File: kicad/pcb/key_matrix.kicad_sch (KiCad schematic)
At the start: 38 parts, among them SW1 EC_SW, SW10 EC_SW, SW11 EC_SW, SW12 EC_SW, SW13 EC_SW, SW14 EC_SW, SW15 EC_SW, SW2 EC_SW, SW3 EC_SW, SW35 SW_Push, SW36 Rotary_Encoder_Switch, SW4 EC_SW, SW5 EC_SW, SW6 EC_SW, SW7 EC_SW, SW8 EC_SW, SW9 EC_SW

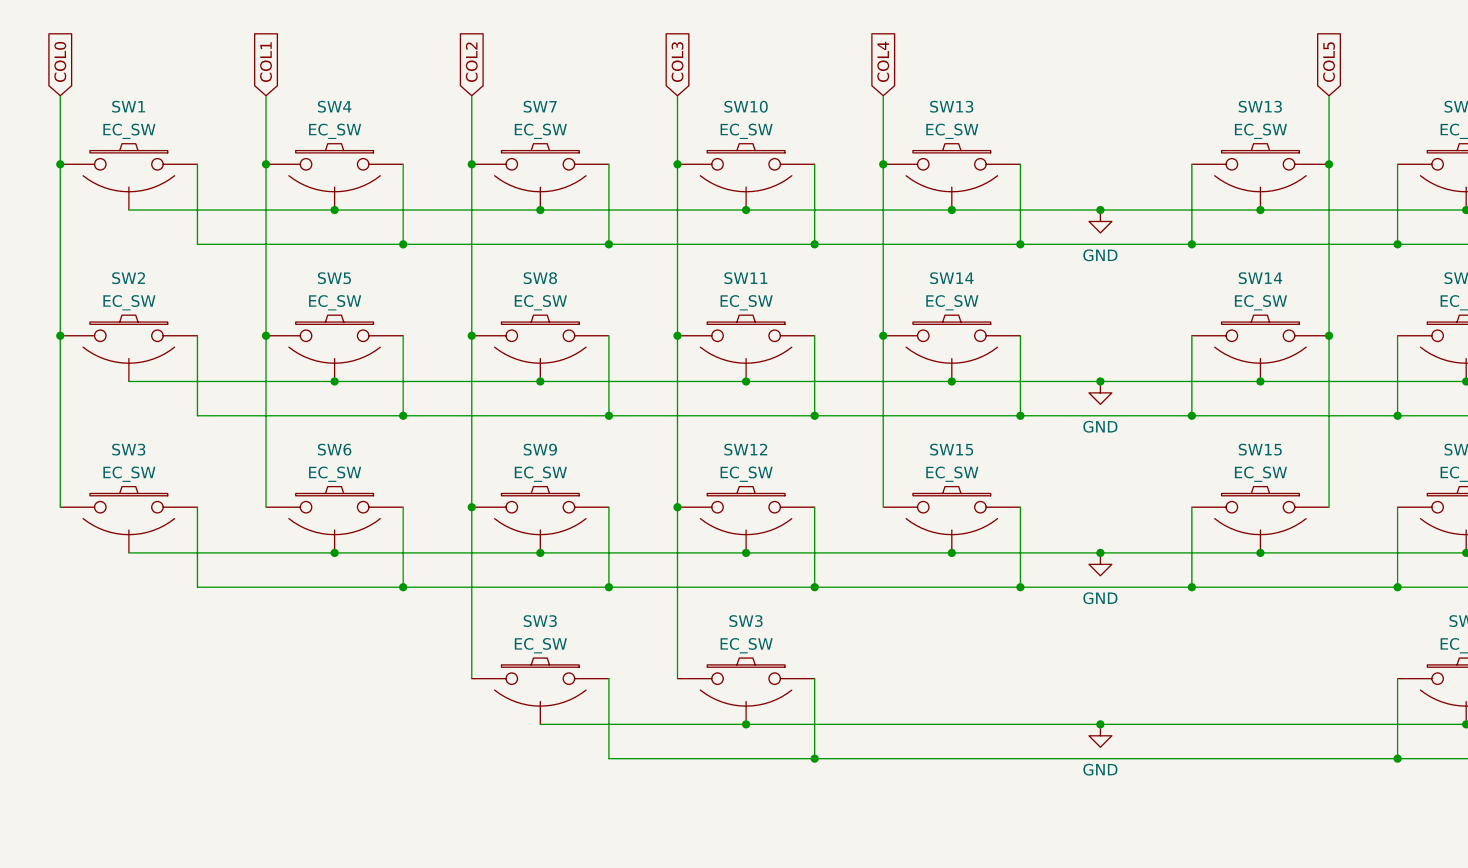
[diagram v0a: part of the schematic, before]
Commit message: rerouted pcb
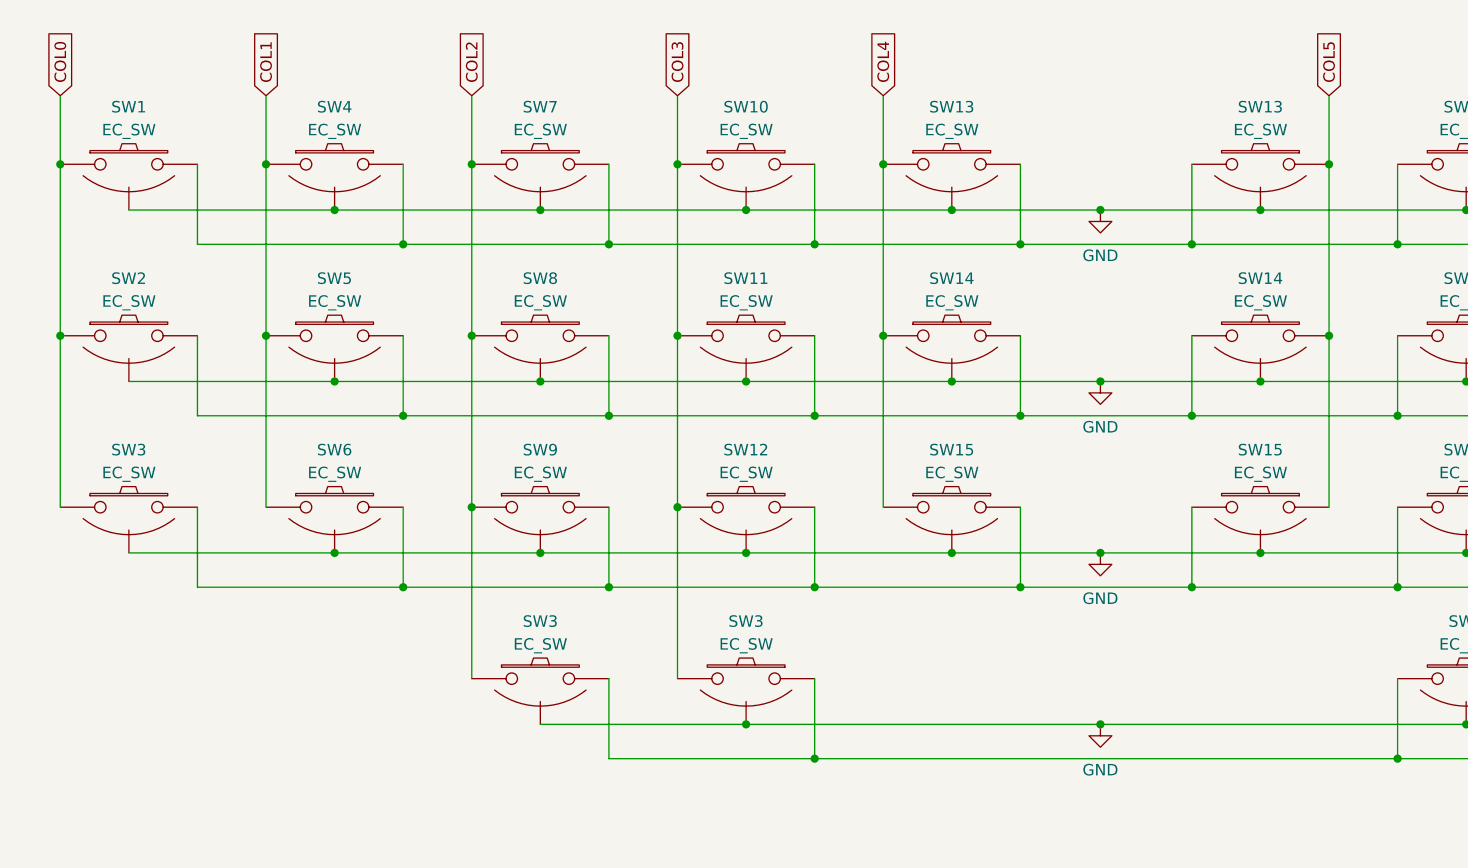
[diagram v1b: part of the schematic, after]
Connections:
- net COL0: now also SW1.1, SW2.1, SW3.1; no longer SW1.2, SW2.2, SW3.2
- net COL1: now also SW4.1, SW5.1, SW6.1; no longer SW4.2, SW5.2, SW6.2
- net COL2: now also SW3.1, SW7.1, SW8.1, SW9.1; no longer SW3.2, SW7.2, SW8.2, SW9.2
- net COL3: now also SW10.1, SW11.1, SW12.1; no longer SW10.2, SW11.2, SW12.2
- net COL4: now also SW13.1, SW14.1, SW15.1; no longer SW13.2, SW14.2, SW15.2
- net COL5: now also SW14.2; no longer SW14.1
- net ROW0: now also SW1.2, SW10.2, SW13.2, SW4.2, SW7.2; no longer SW1.1, SW10.1, SW13.1, SW4.1, SW7.1
- net ROW1: now also SW11.2, SW14.1, SW14.2, SW2.2, SW5.2, SW8.2; no longer SW11.1, SW14.1, SW14.2, SW2.1, SW5.1, SW8.1
- net ROW2: now also SW12.2, SW15.2, SW3.2, SW6.2, SW9.2; no longer SW12.1, SW15.1, SW3.1, SW6.1, SW9.1
- net ROW3: now also SW3.2; no longer SW3.1
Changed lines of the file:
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@@
     )
   )
-  (symbol (lib_id "cipulot_parts:EC_SW") (at 133.985 39.37 0) (mirror y) (unit 1)
+  (symbol (lib_id "cipulot_parts:EC_SW") (at 133.985 39.37 0) (unit 1)
     (in_bom no) (on_board yes) (dnp no)
     (property "Reference" "SW13" (at 133.985 33.02 0)
@@
     )
   )
-  (symbol (lib_id "cipulot_parts:EC_SW") (at 133.985 58.42 0) (mirror y) (unit 1)
+  (symbol (lib_id "cipulot_parts:EC_SW") (at 133.985 58.42 0) (unit 1)
     (in_bom no) (on_board yes) (dnp no)
     (property "Reference" "SW14" (at 133.985 52.07 0)
@@
     )
   )
-  (symbol (lib_id "cipulot_parts:EC_SW") (at 65.405 58.42 0) (mirror y) (unit 1)
+  (symbol (lib_id "cipulot_parts:EC_SW") (at 65.405 58.42 0) (unit 1)
     (in_bom no) (on_board yes) (dnp no)
     (property "Reference" "SW5" (at 65.405 52.07 0)
@@
     )
   )
-  (symbol (lib_id "cipulot_parts:EC_SW") (at 88.265 77.47 0) (mirror y) (unit 1)
+  (symbol (lib_id "cipulot_parts:EC_SW") (at 88.265 77.47 0) (unit 1)
     (in_bom no) (on_board yes) (dnp no)
     (property "Reference" "SW9" (at 88.265 71.12 0)
@@
     )
   )
-  (symbol (lib_id "cipulot_parts:EC_SW") (at 88.265 58.42 0) (mirror y) (unit 1)
+  (symbol (lib_id "cipulot_parts:EC_SW") (at 88.265 58.42 0) (unit 1)
     (in_bom no) (on_board yes) (dnp no)
     (property "Reference" "SW8" (at 88.265 52.07 0)
@@
     )
   )
-  (symbol (lib_id "cipulot_parts:EC_SW") (at 88.265 96.52 0) (mirror y) (unit 1)
+  (symbol (lib_id "cipulot_parts:EC_SW") (at 88.265 96.52 0) (unit 1)
     (in_bom no) (on_board yes) (dnp no)
     (property "Reference" "SW3" (at 88.265 90.17 0)
@@
     )
   )
-  (symbol (lib_id "cipulot_parts:EC_SW") (at 111.125 58.42 0) (mirror y) (unit 1)
+  (symbol (lib_id "cipulot_parts:EC_SW") (at 111.125 58.42 0) (unit 1)
     (in_bom no) (on_board yes) (dnp no)
     (property "Reference" "SW11" (at 111.125 52.07 0)
@@
     )
   )
-  (symbol (lib_id "cipulot_parts:EC_SW") (at 88.265 39.37 0) (mirror y) (unit 1)
+  (symbol (lib_id "cipulot_parts:EC_SW") (at 88.265 39.37 0) (unit 1)
     (in_bom no) (on_board yes) (dnp no)
     (property "Reference" "SW7" (at 88.265 33.02 0)
@@
     )
   )
-  (symbol (lib_id "cipulot_parts:EC_SW") (at 42.545 77.47 0) (mirror y) (unit 1)
+  (symbol (lib_id "cipulot_parts:EC_SW") (at 42.545 77.47 0) (unit 1)
     (in_bom no) (on_board yes) (dnp no)
     (property "Reference" "SW3" (at 42.545 71.12 0)
@@
     )
   )
-  (symbol (lib_id "cipulot_parts:EC_SW") (at 168.275 58.42 0) (mirror y) (unit 1)
+  (symbol (lib_id "cipulot_parts:EC_SW") (at 168.275 58.42 0) (unit 1)
     (in_bom no) (on_board yes) (dnp no)
     (property "Reference" "SW14" (at 168.275 52.07 0)
@@
     )
   )
-  (symbol (lib_id "cipulot_parts:EC_SW") (at 65.405 39.37 0) (mirror y) (unit 1)
+  (symbol (lib_id "cipulot_parts:EC_SW") (at 65.405 39.37 0) (unit 1)
     (in_bom no) (on_board yes) (dnp no)
     (property "Reference" "SW4" (at 65.405 33.02 0)
@@
     )
   )
-  (symbol (lib_id "cipulot_parts:EC_SW") (at 133.985 77.47 0) (mirror y) (unit 1)
+  (symbol (lib_id "cipulot_parts:EC_SW") (at 133.985 77.47 0) (unit 1)
     (in_bom no) (on_board yes) (dnp no)
     (property "Reference" "SW15" (at 133.985 71.12 0)
@@
     )
   )
-  (symbol (lib_id "cipulot_parts:EC_SW") (at 42.545 39.37 0) (mirror y) (unit 1)
+  (symbol (lib_id "cipulot_parts:EC_SW") (at 42.545 39.37 0) (unit 1)
     (in_bom no) (on_board yes) (dnp no)
     (property "Reference" "SW1" (at 42.545 33.02 0)
@@
     )
   )
-  (symbol (lib_id "cipulot_parts:EC_SW") (at 42.545 58.42 0) (mirror y) (unit 1)
+  (symbol (lib_id "cipulot_parts:EC_SW") (at 42.545 58.42 0) (unit 1)
     (in_bom no) (on_board yes) (dnp no)
     (property "Reference" "SW2" (at 42.545 52.07 0)
@@
     )
   )
-  (symbol (lib_id "cipulot_parts:EC_SW") (at 111.125 77.47 0) (mirror y) (unit 1)
+  (symbol (lib_id "cipulot_parts:EC_SW") (at 111.125 77.47 0) (unit 1)
     (in_bom no) (on_board yes) (dnp no)
     (property "Reference" "SW12" (at 111.125 71.12 0)
@@
     )
   )
-  (symbol (lib_id "cipulot_parts:EC_SW") (at 111.125 39.37 0) (mirror y) (unit 1)
+  (symbol (lib_id "cipulot_parts:EC_SW") (at 111.125 39.37 0) (unit 1)
     (in_bom no) (on_board yes) (dnp no)
     (property "Reference" "SW10" (at 111.125 33.02 0)
@@
     )
   )
-  (symbol (lib_id "cipulot_parts:EC_SW") (at 65.405 77.47 0) (mirror y) (unit 1)
+  (symbol (lib_id "cipulot_parts:EC_SW") (at 65.405 77.47 0) (unit 1)
     (in_bom no) (on_board yes) (dnp no)
     (property "Reference" "SW6" (at 65.405 71.12 0)
